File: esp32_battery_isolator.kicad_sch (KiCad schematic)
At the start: 98 parts, among them J1 Conn_01x03_Male, J2 USB_C_Receptacle_USB2.0, Q1 MMBT3904, Q10 MMBT3904, Q11 MMBT3906, Q12 AONR21357, Q13 MMBT3904, Q14 MMBT3904, Q15 MMBT3904, Q16 MMBT3906, Q17 MMBT3904, Q18 AONR21357, Q19 MMBT3904, Q2 MMBT3904, Q20 MMBT3906, Q21 AONR21357, Q3 MMBT3906, Q4 HSBA100P03, Q5 HSBA100P03, Q6 HSBA100P03, Q7 HSBA100P03, Q8 MMBT3904, Q9 MMBT3904, SW1 C620183, SW2 C620183, U1 ESP32-WROOM-32D, U10 INA219BxDCN, U2 INA219BxDCN, U3 INA219BxDCN, U4 INA219BxDCN, U5 XL1509_SOP8, U6 CH340N, U7 INA219BxDCN, U8 ADC128D818, U9 INA219BxDCN

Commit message: small schematic tweaks
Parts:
- Q11, Q16, Q20: lcsc_part_number https://datasheet.lcsc.com/lcsc/1811141238_Shikues-MMBT3906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 -> C111114
- U10, U2, U3, U4, U7, U9: lcsc_part_number (none) -> C2155693
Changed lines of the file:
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@@
       (effects (font (size 1.27 1.27) italic) (justify left) hide)
     )
-    (property "Datasheet" "C111114" (id 3) (at 237.998 68.58 0)
+    (property "Datasheet" "https://datasheet.lcsc.com/lcsc/1811141238_Shikues-MMBT3906_C111114.pdf" (id 3) (at 237.998 68.58 0)
       (effects (font (size 1.27 1.27)) (justify left) hide)
     )
-    (property "lcsc_part_number" "https://datasheet.lcsc.com/lcsc/1811141238_Shikues-MMBT3906_C111114.pdf" (id 4) (at 237.998 68.58 0)
+    (property "lcsc_part_number" "C111114" (id 4) (at 237.998 68.58 0)
       (effects (font (size 1.27 1.27)) hide)
     )
@@
       (effects (font (size 1.27 1.27) italic) (justify left) hide)
     )
-    (property "Datasheet" "C111114" (id 3) (at 347.091 68.834 0)
+    (property "Datasheet" "https://datasheet.lcsc.com/lcsc/1811141238_Shikues-MMBT3906_C111114.pdf" (id 3) (at 347.091 68.834 0)
       (effects (font (size 1.27 1.27)) (justify left) hide)
     )
-    (property "lcsc_part_number" "https://datasheet.lcsc.com/lcsc/1811141238_Shikues-MMBT3906_C111114.pdf" (id 4) (at 347.091 68.834 0)
+    (property "lcsc_part_number" "C111114" (id 4) (at 347.091 68.834 0)
       (effects (font (size 1.27 1.27)) hide)
     )
@@
       (effects (font (size 1.27 1.27) italic) (justify left) hide)
     )
-    (property "Datasheet" "C111114" (id 3) (at 330.581 133.223 0)
+    (property "Datasheet" "https://datasheet.lcsc.com/lcsc/1811141238_Shikues-MMBT3906_C111114.pdf" (id 3) (at 330.581 133.223 0)
       (effects (font (size 1.27 1.27)) (justify left) hide)
     )
-    (property "lcsc_part_number" "https://datasheet.lcsc.com/lcsc/1811141238_Shikues-MMBT3906_C111114.pdf" (id 4) (at 330.581 133.223 0)
+    (property "lcsc_part_number" "C111114" (id 4) (at 330.581 133.223 0)
       (effects (font (size 1.27 1.27)) hide)
     )
@@
     )
     (property "Datasheet" "http://www.ti.com/lit/ds/symlink/ina219.pdf" (id 3) (at 290.068 58.42 0)
+      (effects (font (size 1.27 1.27)) hide)
+    )
+    (property "lcsc_part_number" "C2155693" (id 4) (at 281.178 55.88 0)
       (effects (font (size 1.27 1.27)) hide)
     )
@@
       (effects (font (size 1.27 1.27)) hide)
     )
+    (property "lcsc_part_number" "C2155693" (id 4) (at 96.52 78.105 0)
+      (effects (font (size 1.27 1.27)) hide)
+    )
     (pin "1")
     (pin "2")
@@
       (effects (font (size 1.27 1.27)) hide)
     )
+    (property "lcsc_part_number" "C2155693" (id 4) (at 373.761 118.618 0)
+      (effects (font (size 1.27 1.27)) hide)
+    )
     (pin "1")
     (pin "2")
@@
       (effects (font (size 1.27 1.27)) hide)
     )
+    (property "lcsc_part_number" "C2155693" (id 4) (at 168.275 120.65 0)
+      (effects (font (size 1.27 1.27)) hide)
+    )
     (pin "1")
     (pin "2")
@@
     )
     (property "Datasheet" "http://www.ti.com/lit/ds/symlink/ina219.pdf" (id 3) (at 399.161 58.674 0)
+      (effects (font (size 1.27 1.27)) hide)
+    )
+    (property "lcsc_part_number" "C2155693" (id 4) (at 390.271 56.134 0)
       (effects (font (size 1.27 1.27)) hide)
     )
@@
       (effects (font (size 1.27 1.27)) hide)
     )
+    (property "lcsc_part_number" "C2155693" (id 4) (at 168.021 58.166 0)
+      (effects (font (size 1.27 1.27)) hide)
+    )

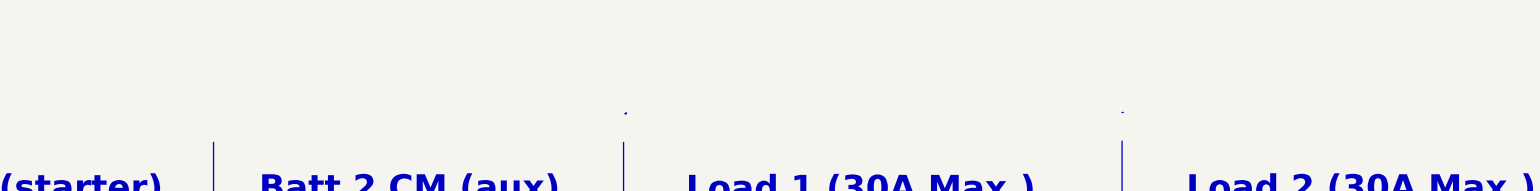
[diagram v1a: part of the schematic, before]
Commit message: WIP
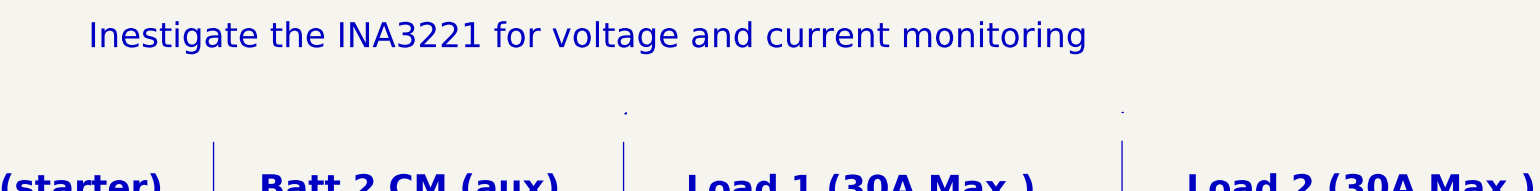
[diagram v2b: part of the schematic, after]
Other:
- note added: "Inestigate the INA3221 for voltage and current monitoring"
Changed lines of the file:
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@@
     (effects (font (size 1.27 1.27)) (justify left bottom))
+  )
+  (text "Inestigate the INA3221 for voltage and current monitoring"
+    (at 94.615 -6.35 0)
+    (effects (font (size 5.08 5.08)) (justify left bottom))
   )
   (text "ESP-32 Microcontroller" (at 19.3294 160.782 0)

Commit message: Changed from push pull to independent pull up and pull down mosfets
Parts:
- removed Q10, Q19, Q2: MMBT3904, Package_TO_SOT_SMD:SOT-23, symbol Transistor_BJT:MMBT3904
- removed Q11, Q20, Q3: MMBT3906, Package_TO_SOT_SMD:SOT-23, symbol Transistor_BJT:MMBT3906
- added Q10, Q11, Q2: Q_PMOS_GSD, Package_TO_SOT_SMD:SOT-23, symbol Device:Q_PMOS_GSD
- added Q19, Q20, Q3: 2N7002, Package_TO_SOT_SMD:SOT-23, symbol Transistor_FET:2N7002
- added R13, R17, R24: 5k, Resistor_SMD:R_0603_1608Metric, symbol Device:R_Small
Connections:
- net B1ON: now also U1.12 (IO27), Q3.1 (G); no longer R1.1, U1.8 (IO32)
- net COM: now also Q10.2 (S), Q11.2 (S), Q2.2 (S), R13.2, R17.2, R24.2
- net D: no longer Q4.2 (D), Q5.2 (D)
- net G: now also Q2.3 (D), Q3.3 (D)
- net GND: now also Q19.2 (S), Q20.2 (S), Q3.2 (S)
- net L1ON: now also U1.23 (IO15), Q19.1 (G); no longer R15.1, U1.13 (IO14)
- net L2ON: now also U1.29 (IO5), Q20.1 (G); no longer R21.1, U1.16 (IO13)
- net at Q9.3 (C): now also Q10.1 (G), R17.1
- net at Q12.1 (G): now also Q10.3 (D), Q19.3 (D)
- net at Q1.3 (C): now also Q2.1 (G), R13.1
- net at Q17.3 (C): now also Q11.1 (G), R24.1
- net at Q21.1 (G): now also Q11.3 (D), Q20.3 (D)
- new net: Q4.2 (D), Q5.2 (D)
- new net B1OFF: R1.1, U1.8 (IO32)
- new net L1OFF: R15.1, U1.13 (IO14)
- new net L2OFF: R21.1, U1.16 (IO13)
- no-connect marks 27 -> 24
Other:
- moved on the sheet: BZ1, C1, C10, C11, C12, C13, C14, C15, C16, C17, C18, C2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

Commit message: More cleanup
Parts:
- added C19: 100uF(220uF), Capacitor_SMD:C_Elec_6.3x5.4, symbol Device:CP_Small
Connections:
- net COM: now also C19.1
- net D: now also Q4.2 (D), Q5.2 (D)
- net GND: now also C19.2
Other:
- moved on the sheet: C12, C4, C6, C7, C8, C9, D1, D2, D3, D4, D5, H1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
